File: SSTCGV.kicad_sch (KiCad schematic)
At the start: 46 parts, among them IC1 ATTINY13-20PU, J1-1 INPUT 1, J1-2 INPUT 2, J2 COILS, J3 POWER, J4 OPT, Q1 IRLZ44N, Q2 IRLZ44N, Q3 IRLZ44N, SW1 SW_Push_DPDT, U1 EL817, U2 L78L05

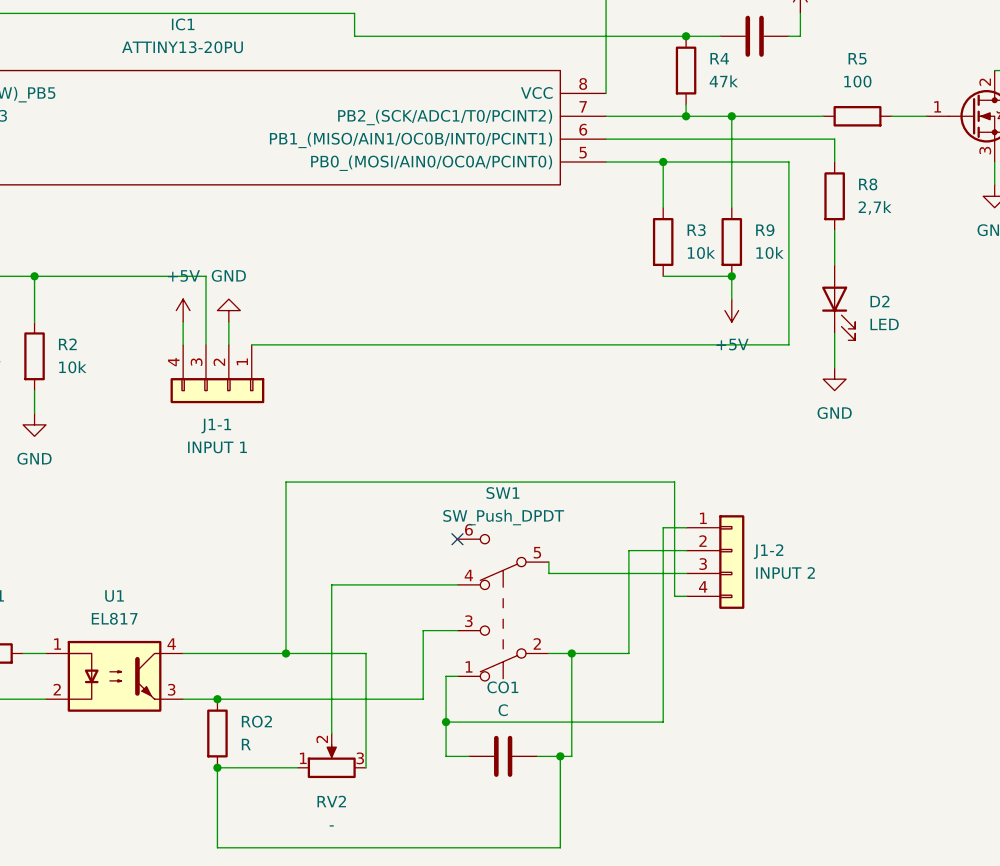
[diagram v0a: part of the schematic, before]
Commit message: woking on pcb
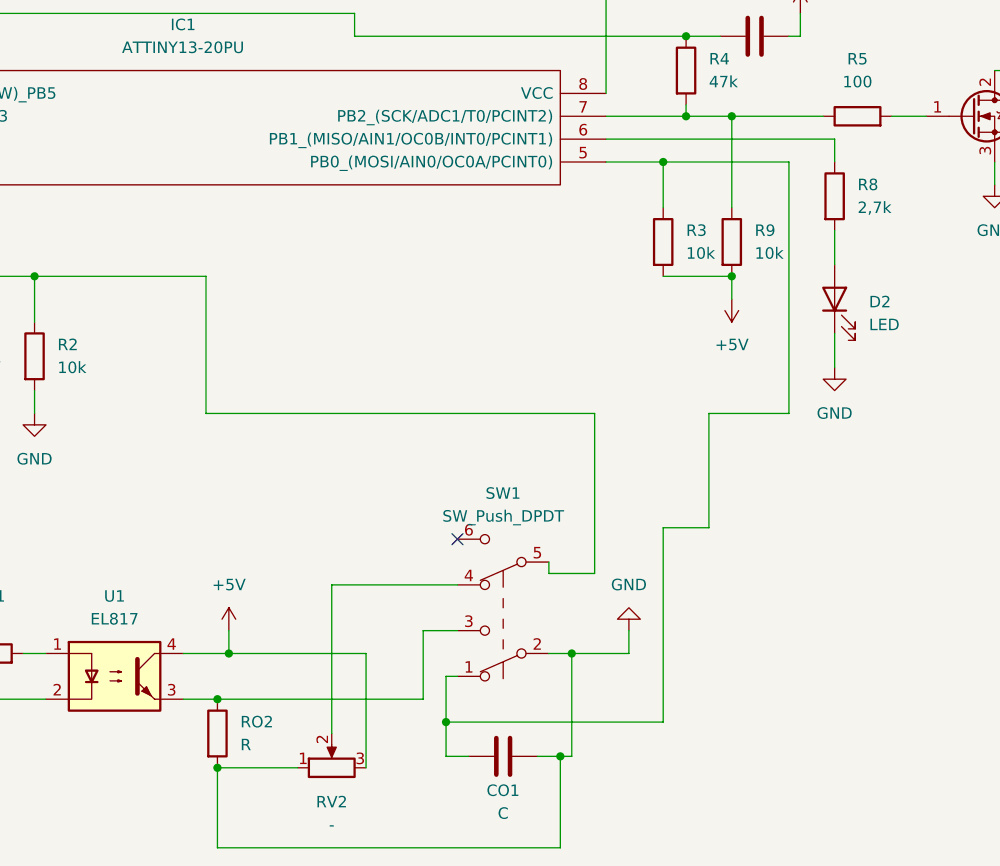
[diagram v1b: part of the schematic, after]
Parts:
- removed J1-1: INPUT 1, Connector_PinSocket_2.54mm:PinSocket_1x04_P2.54mm_Vertical, symbol Connector_Generic:Conn_01x04
- removed J1-2: INPUT 2, Connector_PinSocket_2.54mm:PinSocket_1x04_P2.54mm_Vertical, symbol Connector_Generic:Conn_01x04
- D2: footprint LED_THT:LED_D5.0mm-3_Horizontal_O3.81mm_Z3.0mm -> LED_THT:LED_D5.0mm-3
- R1: footprint Resistor_THT:R_Axial_DIN0411_L9.9mm_D3.6mm_P15.24mm_Horizontal -> Resistor_THT:R_Axial_DIN0309_L9.0mm_D3.2mm_P5.08mm_Vertical
- R2, R3, R4, R5, R6, R8, R9, RO1, RO2: footprint Resistor_THT:R_Axial_DIN0411_L9.9mm_D3.6mm_P15.24mm_Horizontal -> Resistor_THT:R_Axial_DIN0411_L9.9mm_D3.6mm_P7.62mm_Vertical
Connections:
- net +5V: now also RV2.3, U1.4
- net GND: now also CO1.2, RO2.2, RV2.1, SW1.2 (B)
- net at C3.1, IC1.3 ((PCINT4/ADC2)_PB4), R2.1: now also SW1.5 (B)
- net at IC1.5 (PB0_(MOSI/AIN0/OC0A/PCINT0)), R3.1: now also CO1.1, SW1.1 (A)
